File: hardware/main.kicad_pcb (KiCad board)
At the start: 2 copper layers, 42 x 55 mm, 10 parts

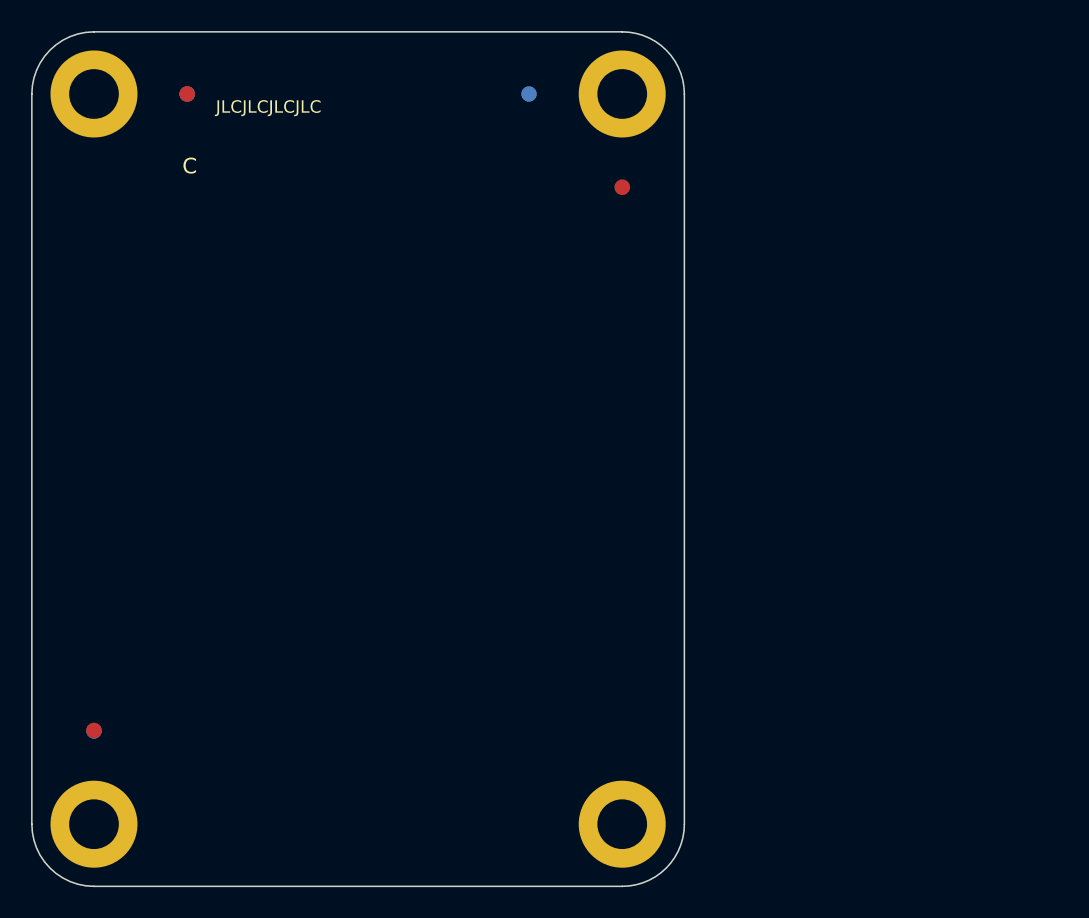
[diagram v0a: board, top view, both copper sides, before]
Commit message: finish pcb
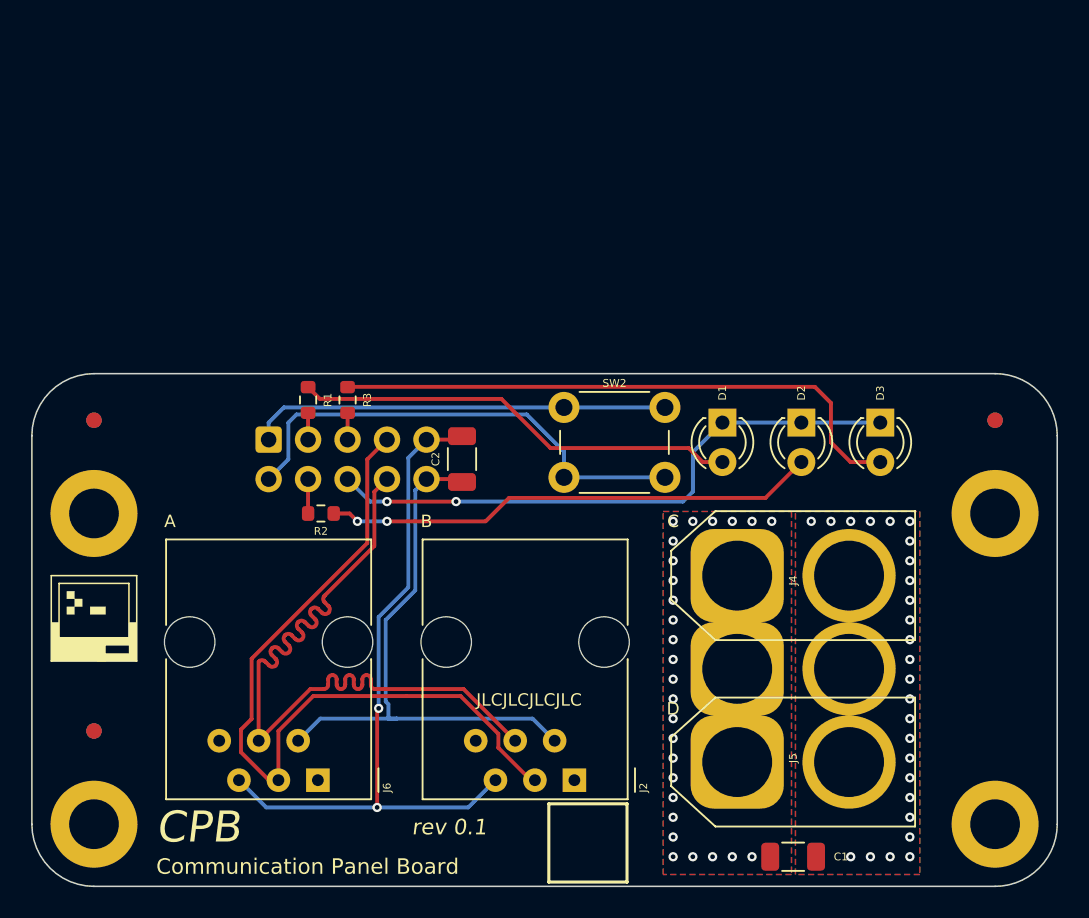
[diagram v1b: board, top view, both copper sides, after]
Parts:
- added C1: 100n, Capacitor_SMD:C_1206_3216Metric, F.Cu at (49.0, -1.91)
- added C2: 100n, Capacitor_SMD:C_1206_3216Metric, F.Cu at (27.7, -27.5)
- added D1: 204-10SUGD(E), LED_THT:LED_D3.0mm, F.Cu at (44.5, -29.9)
- added D2: 204-10UYD(Y), LED_THT:LED_D3.0mm, F.Cu at (49.5, -29.9)
- added D3: 204-10SURD(R), LED_THT:LED_D3.0mm, F.Cu at (54.6, -29.9)
- added J1: DS1013-10S, Connector_IDC:IDC-Header_2x05_P2.54mm_Vertical, B.Cu at (15.2, -28.8)
- added J2: KH-9752-6P6C, MAS_Package_std:RJ12_Vertical, F.Cu at (34.9, -6.83)
- added J3: XT60, MAS_Package_nostd:AMASS_XT60-F_1x02_P7.20mm_Vertical, B.Cu at (45.4, -14.0)
- added J4: XT60, MAS_Package_nostd:AMASS_XT60-M_1x02_P7.20mm_Vertical, F.Cu at (45.4, -20.0)
- added J5: XT60, MAS_Package_nostd:AMASS_XT60-F_1x02_P7.20mm_Vertical, F.Cu at (45.4, -8.00)
- added J6: KH-9752-6P6C, MAS_Package_std:RJ12_Vertical, F.Cu at (18.4, -6.83)
- added R1: 1k, Resistor_SMD:R_0603_1608Metric, F.Cu at (17.8, -31.3)
- added R2: 1k, Resistor_SMD:R_0603_1608Metric, F.Cu at (18.6, -24.0)
- added R3: 1k, Resistor_SMD:R_0603_1608Metric, F.Cu at (20.3, -31.3)
- added SW2: TL1105HF160Q, Button_Switch_THT:SW_PUSH_6mm_H13mm, F.Cu at (34.2, -30.8)
- moved FID4 36.6 mm to (62.0, -30.0)
- moved H2 36.1 mm to (62.0, -24.0)
- moved FID1 28.3 mm to (62.0, -30.0)
- moved H4 27.0 mm to (4.00, -24.0)
- moved H3 24.0 mm to (62.0, -4.00)
- moved FID2 21.8 mm to (4.00, -30.0)
- moved FID6 21.8 mm to (4.00, -30.0)
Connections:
- H4 pad 1: GNDREF -> (no net)
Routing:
- net /CANH: track 0.00 -> 50.5 mm
- net /CANL: track 0.00 -> 50.1 mm
- net /CANgnd: track 0.00 -> 45.3 mm, vias 0 -> 2
- net GND: track 0.00 -> 38.5 mm, vias 0 -> 2
- net Net-(D3-A): track 0.00 -> 37.8 mm
- net /CANvcc: track 0.00 -> 37.2 mm
- net Net-(D2-A): track 0.00 -> 31.9 mm, vias 0 -> 2
- net /K2: track 0.00 -> 31.3 mm
- net Net-(D1-A): track 0.00 -> 28.7 mm
- net /K1: track 0.00 -> 27.0 mm
- net /IO2: track 0.00 -> 2.21 mm
- net /IO3: track 0.00 -> 1.73 mm
- net /IO1: track 0.00 -> 1.73 mm
- net Net-(C1-Pad2): vias 0 -> 26
- net Net-(C1-Pad1): vias 0 -> 27
- added copper zone on B.Cu, net Net-(C1-Pad1)
- added copper zone on F.Cu, net Net-(C1-Pad1)
- added copper zone on B.Cu, net Net-(C1-Pad2)
- added copper zone on F.Cu, net Net-(C1-Pad2)
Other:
- board size 42 x 55 mm -> 66 x 33 mm
- board text added: "A"
- board text added: "B"
- board text added: "CPB"
- board text added: "Communication Panel Board"
- board text added: "D"
- board text added: "E"
- board text added: "F"
- board text removed: "TTTT"
- board text removed: "TTTTT"
